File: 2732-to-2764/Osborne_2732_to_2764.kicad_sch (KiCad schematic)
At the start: 4 parts, among them J1 2732_ROM_Socket, J2 2764_ROM, J3 Conn_01x02

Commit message: Updated socket pins
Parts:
- J1: footprint Package_DIP:DIP-24_W15.24mm -> Open2327RomAdapter:DIP-24_W15.24mm-Notch
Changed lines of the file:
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@@
       (effects (font (size 1.27 1.27)))
     )
-    (property "Footprint" "Package_DIP:DIP-24_W15.24mm" (at 93.98 88.9 0)
+    (property "Footprint" "Open2327RomAdapter:DIP-24_W15.24mm-Notch" (at 93.98 88.9 0)
       (effects (font (size 1.27 1.27)) hide)
     )

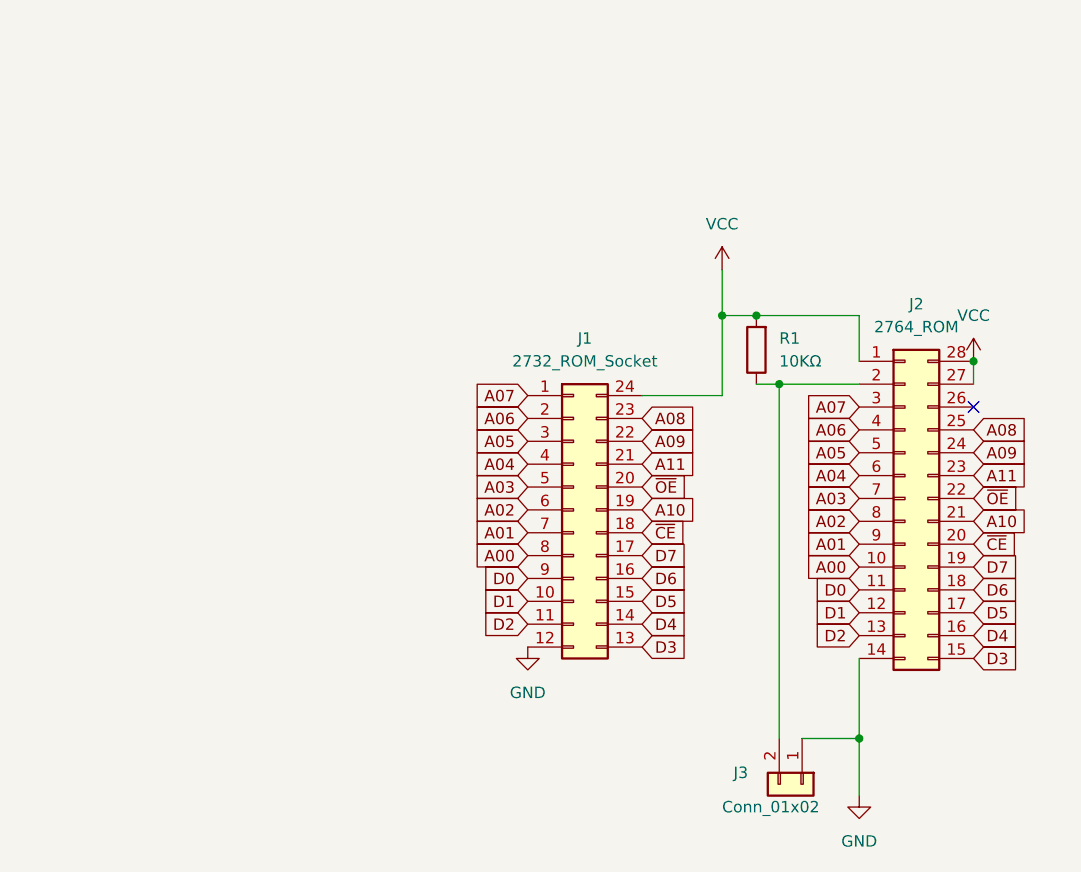
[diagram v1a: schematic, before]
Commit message: Updated to Kicad 8.0.6
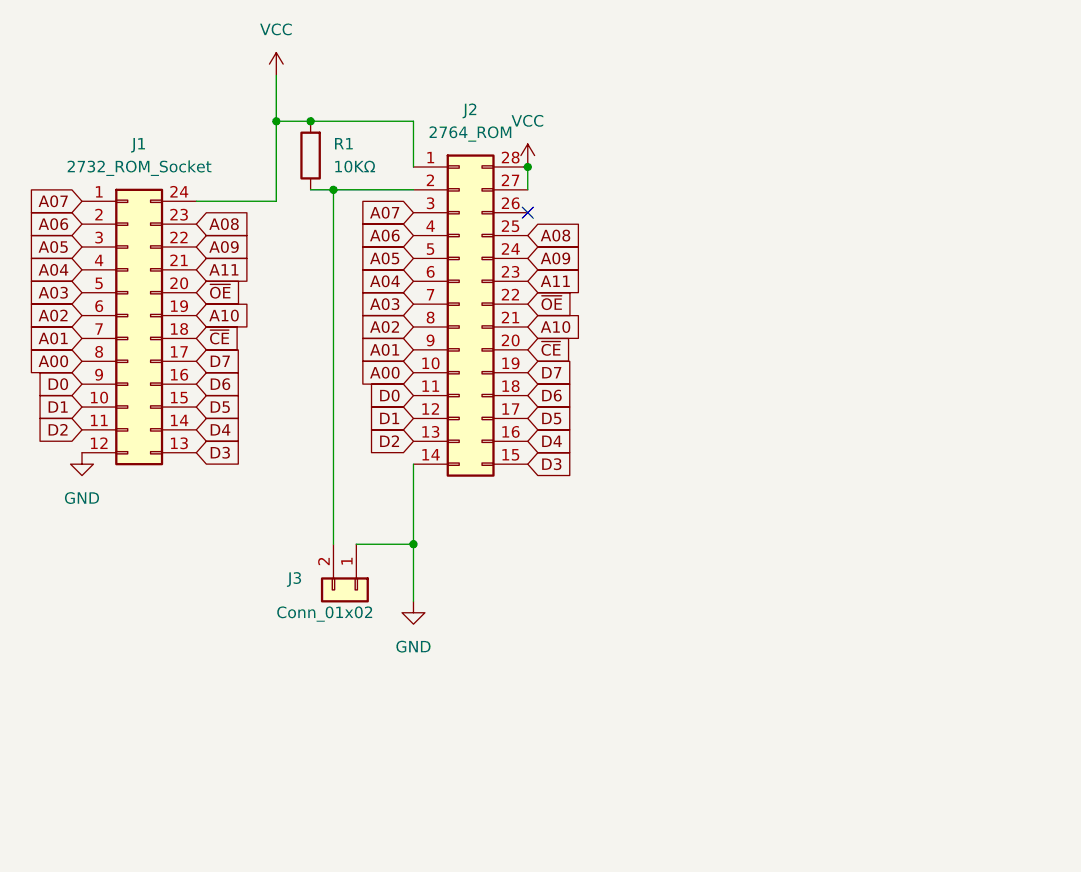
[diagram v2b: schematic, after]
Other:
- company: (none) -> Brett Hallen
- title: (none) -> 2764 to 2732 Adapator
- moved on the sheet: J1, J2, J3, R1
